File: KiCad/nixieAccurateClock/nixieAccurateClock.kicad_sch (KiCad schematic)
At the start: 8 parts, among them J1 Conn_01x02_Pin, J2 Conn_01x02_Pin, J3 Conn_01x02_Pin, SW1 SW_DIP_x08

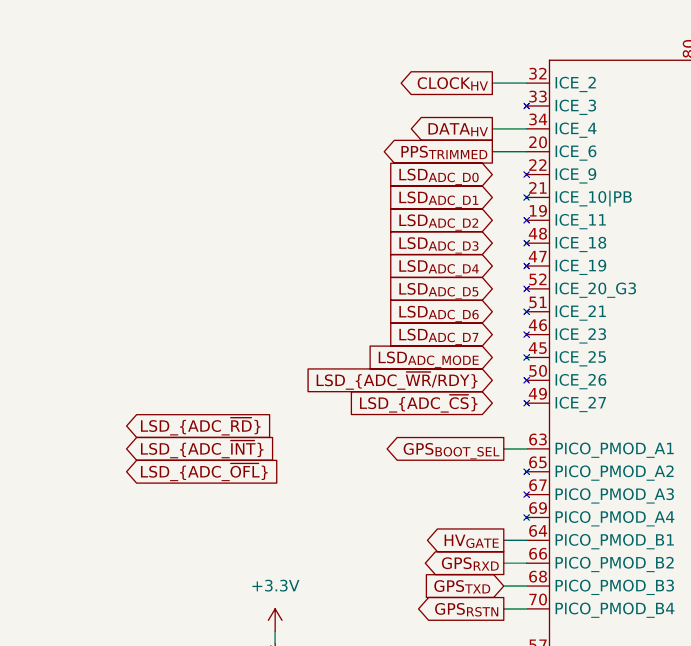
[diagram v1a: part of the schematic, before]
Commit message: give pico iCE better mounting
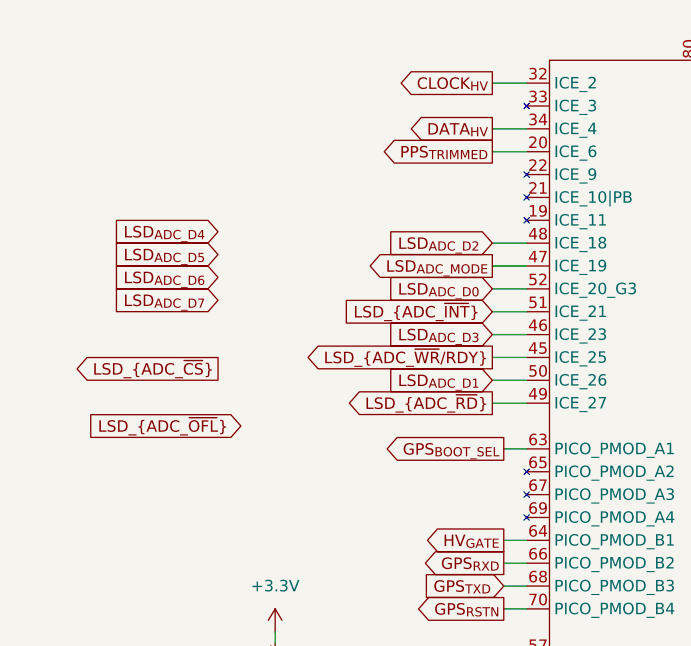
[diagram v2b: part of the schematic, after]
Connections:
- net LSD_{ADC_D0}: now also U1.52 (ICE_20_G3)
- net LSD_{ADC_D1}: now also U1.50 (ICE_26)
- net LSD_{ADC_D2}: now also U1.48 (ICE_18)
- net LSD_{ADC_D3}: now also U1.46 (ICE_23)
- net LSD_{ADC_MODE}: now also U1.47 (ICE_19)
- net LSD_{ADC_~{INT}}: now also U1.51 (ICE_21)
- net LSD_{ADC_~{RD}}: now also U1.49 (ICE_27)
- net LSD_{ADC_~{WR}/RDY}: now also U1.45 (ICE_25)
